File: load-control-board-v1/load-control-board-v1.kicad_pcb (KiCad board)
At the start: 4 copper layers, 100 x 100 mm, 75 parts, among them CN1 3511232BMRS0BNA2, Q1 AO3400A, Q2 AO3400A, Q3 IRFP7530PBF, U1 LM317_SOT-223, U10 OPA188xxDBV, U11 OPA188xxDBV, U12 INA186A1IDCKR, U2 74AHC1G04, U22 TL081HIDR, U3 LM317_SOT-223, U4 TT56145145-1520, U5 REF5025AD, U6 SN74LVC1G123DCUR_C352969, U7 TL081HIDR, U8 OPA188xxDBV, U9 TT56145145-1520

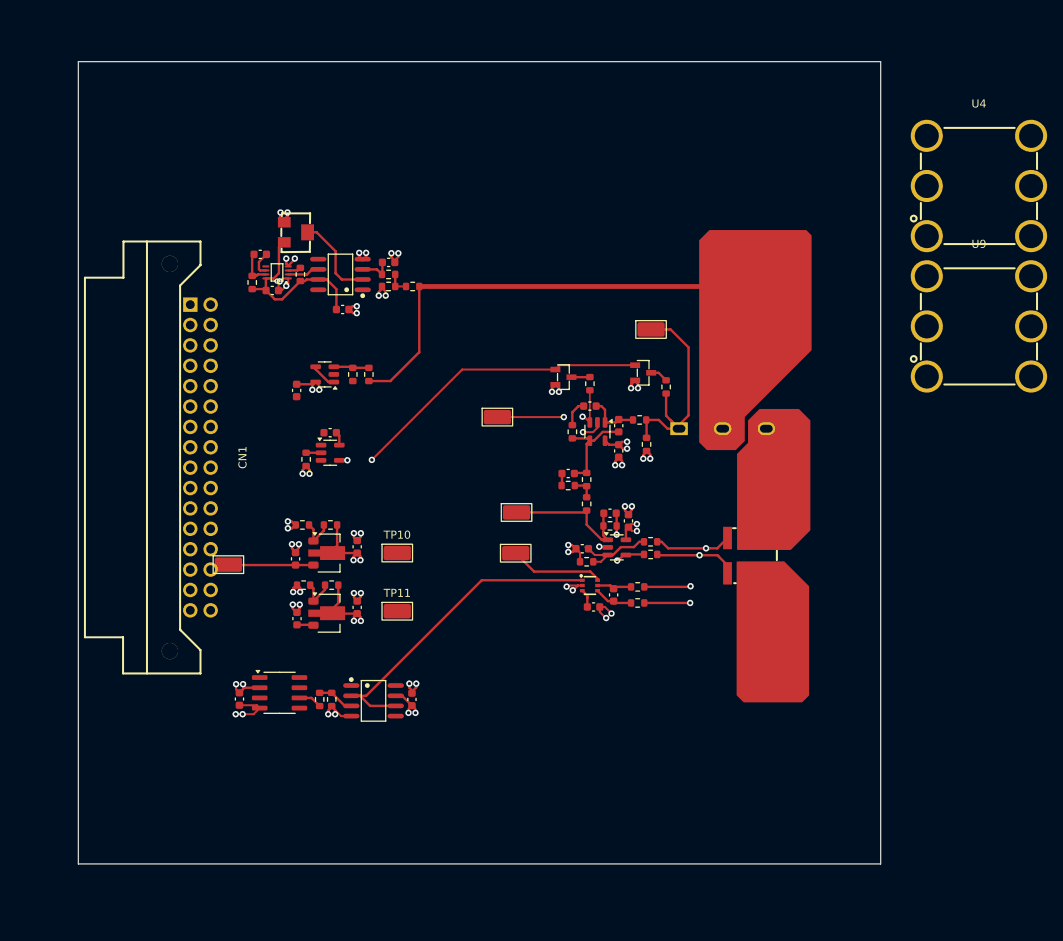
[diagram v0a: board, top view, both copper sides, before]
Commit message: layout before check
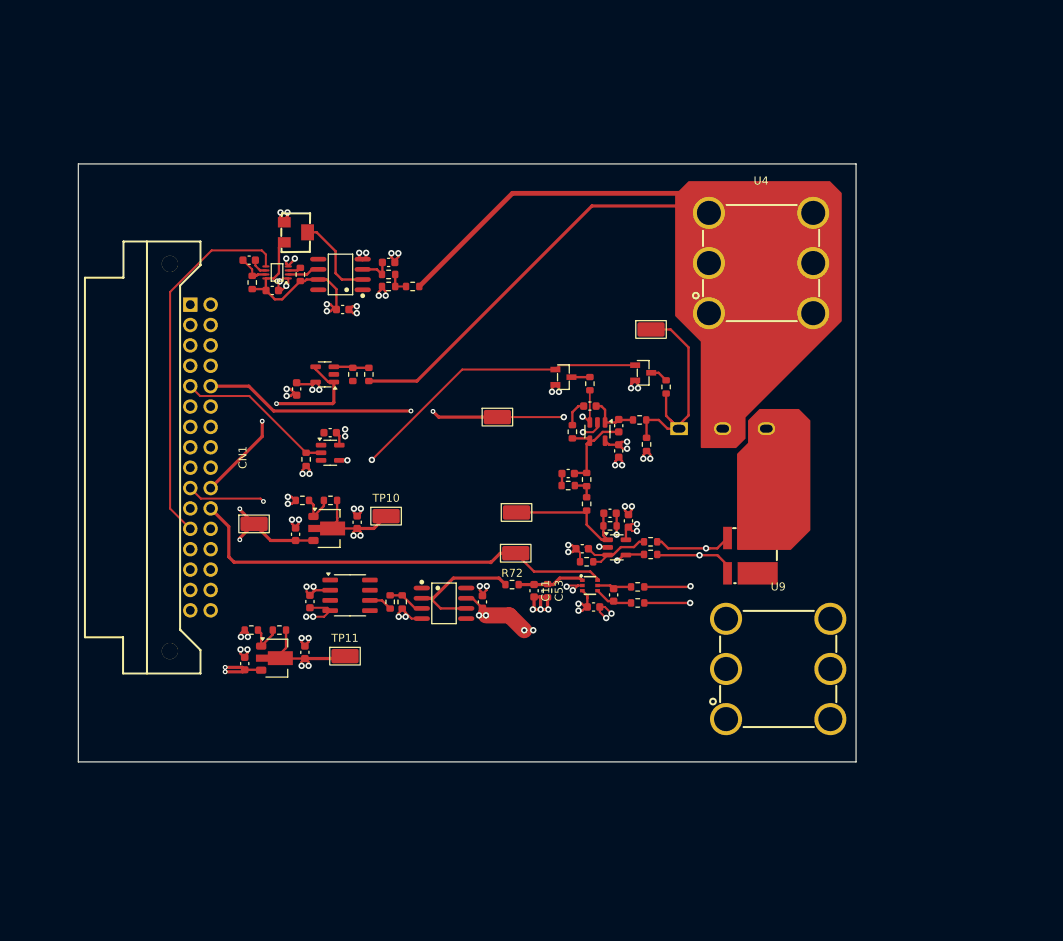
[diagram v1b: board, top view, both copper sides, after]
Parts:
- added C11: 100n, Capacitor_SMD:C_0603_1608Metric, F.Cu at (111.0, 107.7)
- added C53: 1u, Resistor_SMD:R_0603_1608Metric, F.Cu at (112.7, 107.7)
- added R72: 100, Resistor_SMD:R_0603_1608Metric, F.Cu at (108.3, 106.9)
- moved U9 49.5 mm to (141.5, 117.4)
- moved U4 28.8 mm to (139.3, 66.9)
- moved U22 15.0 mm to (99.8, 109.3)
- moved C49 15.0 mm to (104.6, 109.1)
- moved C8 15.0 mm to (83.1, 109.0)
- moved R11 15.0 mm to (93.1, 109.1)
- moved R12 15.0 mm to (94.6, 109.1)
- moved U5 15.0 mm to (88.1, 108.3)
- moved C4 8.59 mm to (75.0, 116.8)
- moved C6 8.59 mm to (82.5, 115.4)
- moved R6 8.59 mm to (79.3, 112.6)
- moved R7 8.59 mm to (75.8, 112.6)
- moved TP11 8.59 mm to (87.5, 115.9)
- moved U3 8.59 mm to (79.0, 116.1)
- moved TP1 6.00 mm to (76.1, 99.4)
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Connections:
- C10 pad 2: 5V -> +5V
- C2 pad 2: 5V -> +5V
- C21 pad 2: 5V -> +5V
- C7 pad 2: 5V -> +5V
- CN1 pad 10: 5V -> +5V
- R13 pad 2: 5V -> +5V
- U12 pad 3: 5V -> +5V
- U2 pad 5: 5V -> +5V
- U6 pad 8: 5V -> +5V
- U7 pad 7: 5V -> +5V
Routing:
- net +12V: track 12.7 -> 74.5 mm, vias 0 -> 4
- net VBUS: track 60.6 -> 122.3 mm
- net +5V: track 104.1 -> 158.9 mm, vias 8 -> 17
- net OV_ALERT: track 0.00 -> 46.3 mm
- net /I_SINK_MON_CH0: track 11.7 -> 55.2 mm
- net +9V: track 107.8 -> 145.3 mm
- net I_CONTROL: track 15.9 -> 53.3 mm, vias 2 -> 4
- net V_BUS_MON: track 3.24 -> 26.9 mm, vias 0 -> 2
- net V_REF: track 39.7 -> 17.9 mm
- net ENABLE: track 1.86 -> 19.7 mm
- net GND: track 71.9 -> 82.5 mm, vias 52 -> 57
- net /ch0/V_REF_FIL: track 0.00 -> 8.38 mm
- net 5V: track 26.7 -> 22.6 mm
- net Net-(U6-Cext): track 3.16 -> 2.23 mm
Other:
- board size 100 x 100 mm -> 96.9 x 74.5 mm
- board text removed: "LDO might need some heat dissapate consideration"
- board text removed: "Move this closer to VBUS power trace Change sample point to the terminal(where the copper wire connect) of VBUS"
- board text removed: "Move voltage reference closer to INA186 Make a guard trace GND for V_REF Place the LPF near INA186"
- board text removed: "Need to change the board edge to match the connector!"

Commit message: layout adjust
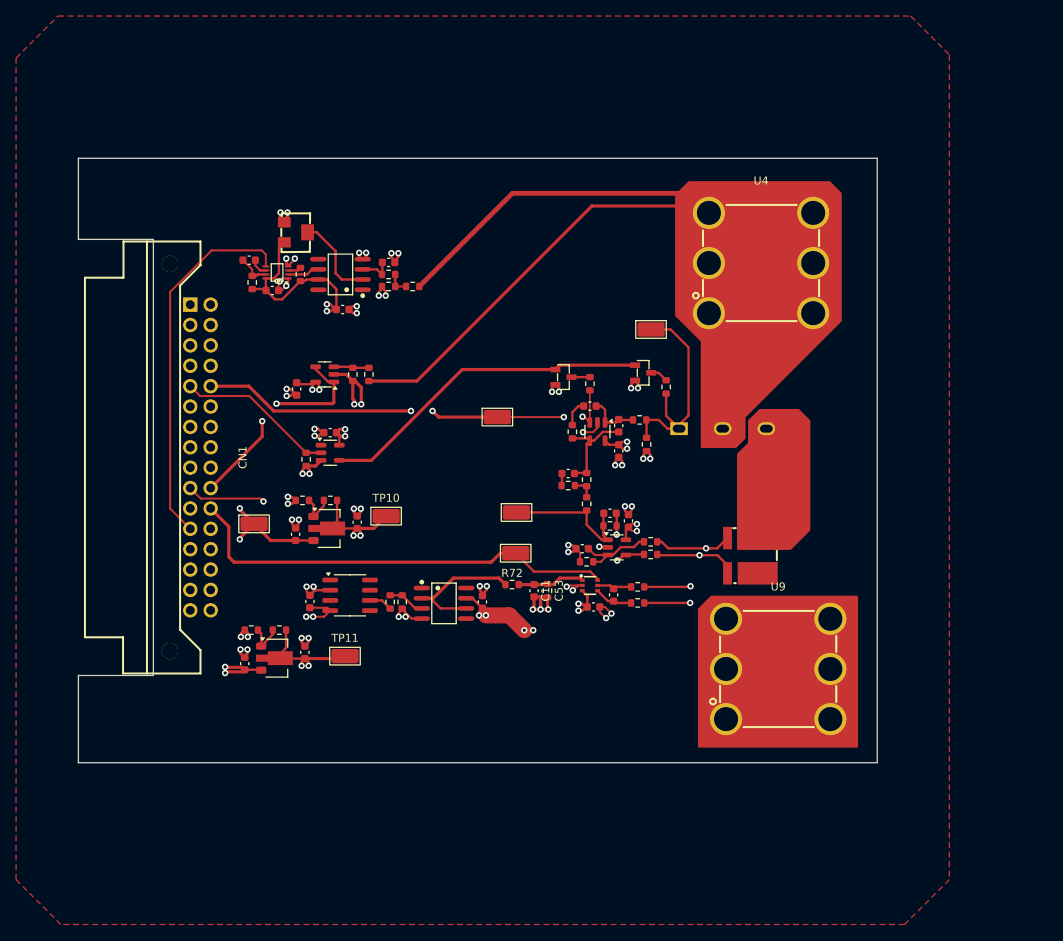
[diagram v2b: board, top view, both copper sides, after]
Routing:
- net GND: track 82.5 -> 96.0 mm, vias 57 -> 61
- net +5V: track 158.9 -> 164.5 mm
- net ~{ENABLE}: track 41.8 -> 41.9 mm, vias 2 -> 0
- added copper zone on F.Cu, net GND
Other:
- board size 96.9 x 74.5 mm -> 99.6 x 75.3 mm
